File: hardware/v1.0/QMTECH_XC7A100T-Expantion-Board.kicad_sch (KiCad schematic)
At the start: 3 parts, among them J1 Conn_01x34, J6 Conn_01x34

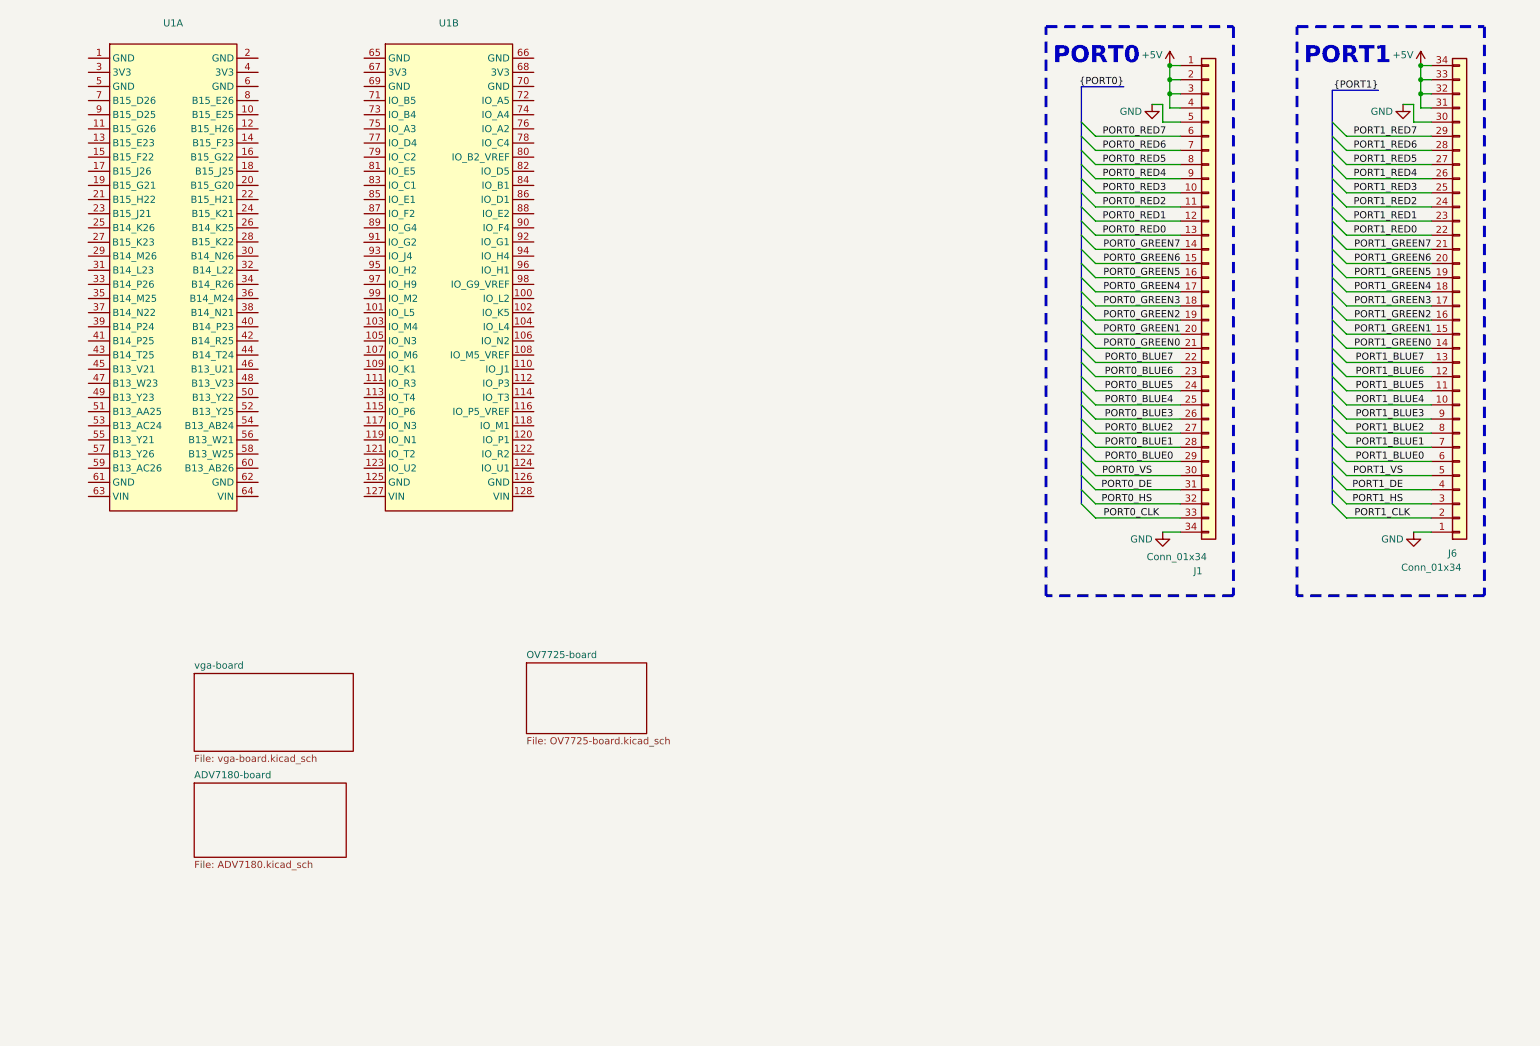
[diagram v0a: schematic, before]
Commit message: backup
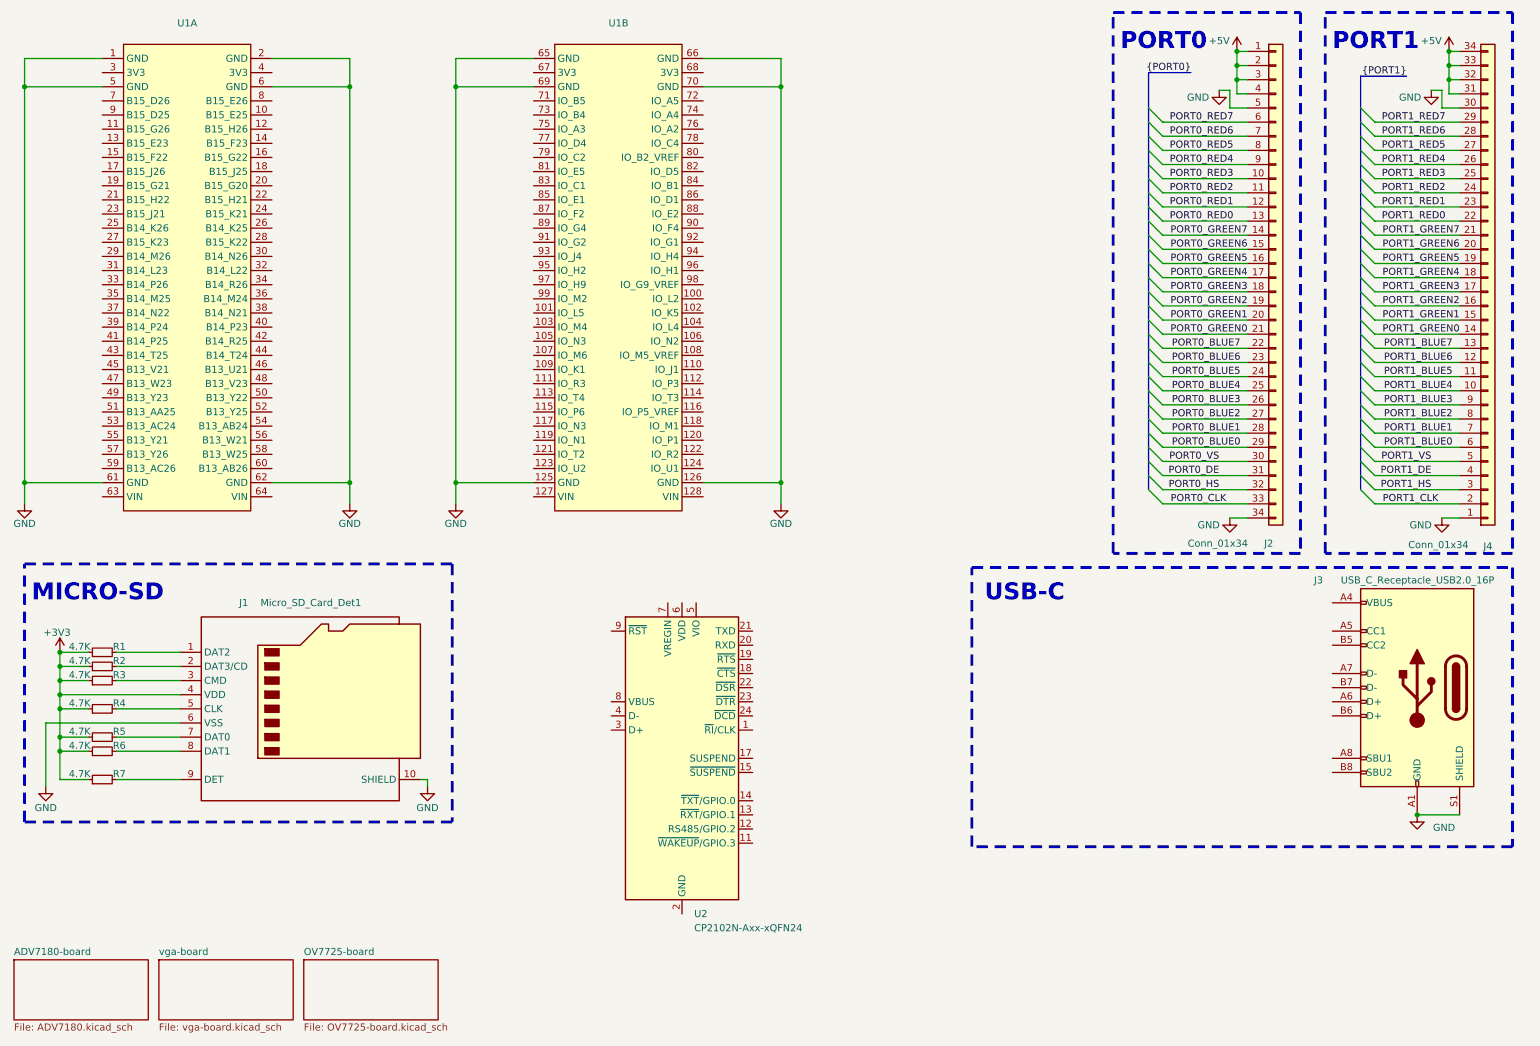
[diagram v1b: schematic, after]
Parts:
- added J1: Micro_SD_Card_Det1, symbol Connector:Micro_SD_Card_Det1
- added J3: USB_C_Receptacle_USB2.0_16P, symbol Connector:USB_C_Receptacle_USB2.0_16P
- added R1, R2, R3, R4, R5, R6, R7: 4.7K, Resistor_SMD:R_0603_1608Metric_Pad0.98x0.95mm_HandSolder, symbol Device:R_Small
- added U2: CP2102N-Axx-xQFN24, Package_DFN_QFN:QFN-24-1EP_4x4mm_P0.5mm_EP2.6x2.6mm, symbol Interface_USB:CP2102N-Axx-xQFN24
- renumbered J1 to J2, J6 to J4
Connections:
- net GND: now also U1.1 (GND), U1.125 (GND), U1.126 (GND), U1.2 (GND), U1.5 (GND), U1.6 (GND), U1.61 (GND), U1.62 (GND), U1.65 (GND), U1.66 (GND), U1.69 (GND), U1.70 (GND), J1.10 (SHIELD), J1.6 (VSS), J3.A1 (GND), J3.A12 (GND), J3.B1 (GND), J3.B12 (GND), J3.S1 (SHIELD)
- new net: U2.2 (GND), U2.25 (GND)
- new net: J1.7 (DAT0), R5.2
- new net: J1.3 (CMD), R3.2
- new net: J1.2 (DAT3/CD), R2.2
- new net: J1.9 (DET), R7.2
- new net: J1.1 (DAT2), R1.2
- new net: J1.5 (CLK), R4.2
- new net: J1.8 (DAT1), R6.2
- new net: J3.A4 (VBUS), J3.A9 (VBUS), J3.B4 (VBUS), J3.B9 (VBUS)
- new net +3V3: J1.4 (VDD), R1.1, R2.1, R3.1, R4.1, R5.1, R6.1, R7.1
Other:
- note added: "MICRO-SD"
- note added: "USB-C"
- moved on the sheet: J2, J4, U1A, U1B
